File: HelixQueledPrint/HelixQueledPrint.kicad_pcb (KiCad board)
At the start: 4 copper layers, 120 parts, among them J1 USB_C_Receptacle_USB2.0_16P, J101 Conn_Coaxial, J601 Screw_Terminal_01x02, SW1 SW_SPST, SW2 SW_SPST, U101 ESP32-C6FHx, U102 BGS12WN6E6327, U202 TPS92201, U302 TPS92201, U402 TPS92201, U502 TPS92201, U601 MB34F, U602 SY8366H, U603 XBL1117, Y1 40MHz

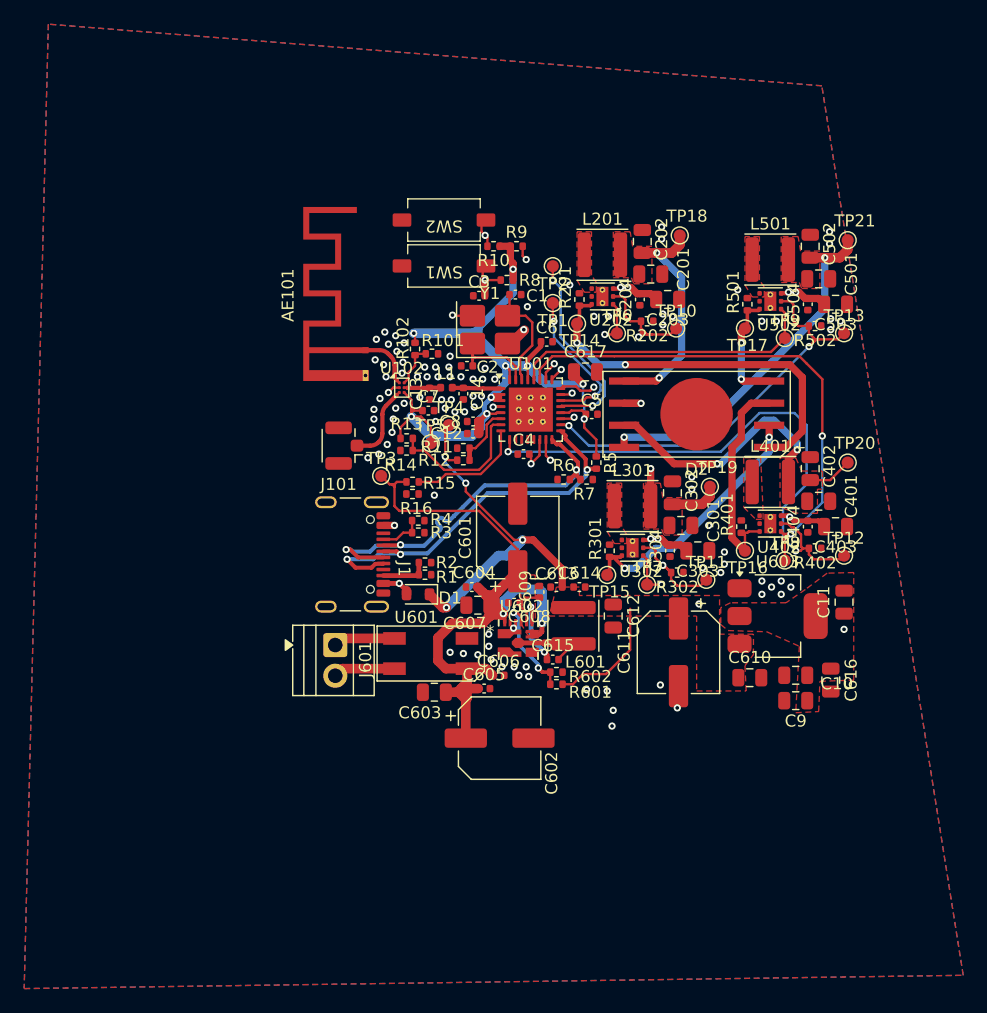
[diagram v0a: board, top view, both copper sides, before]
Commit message: Alles afgerond, geen drc errors meer
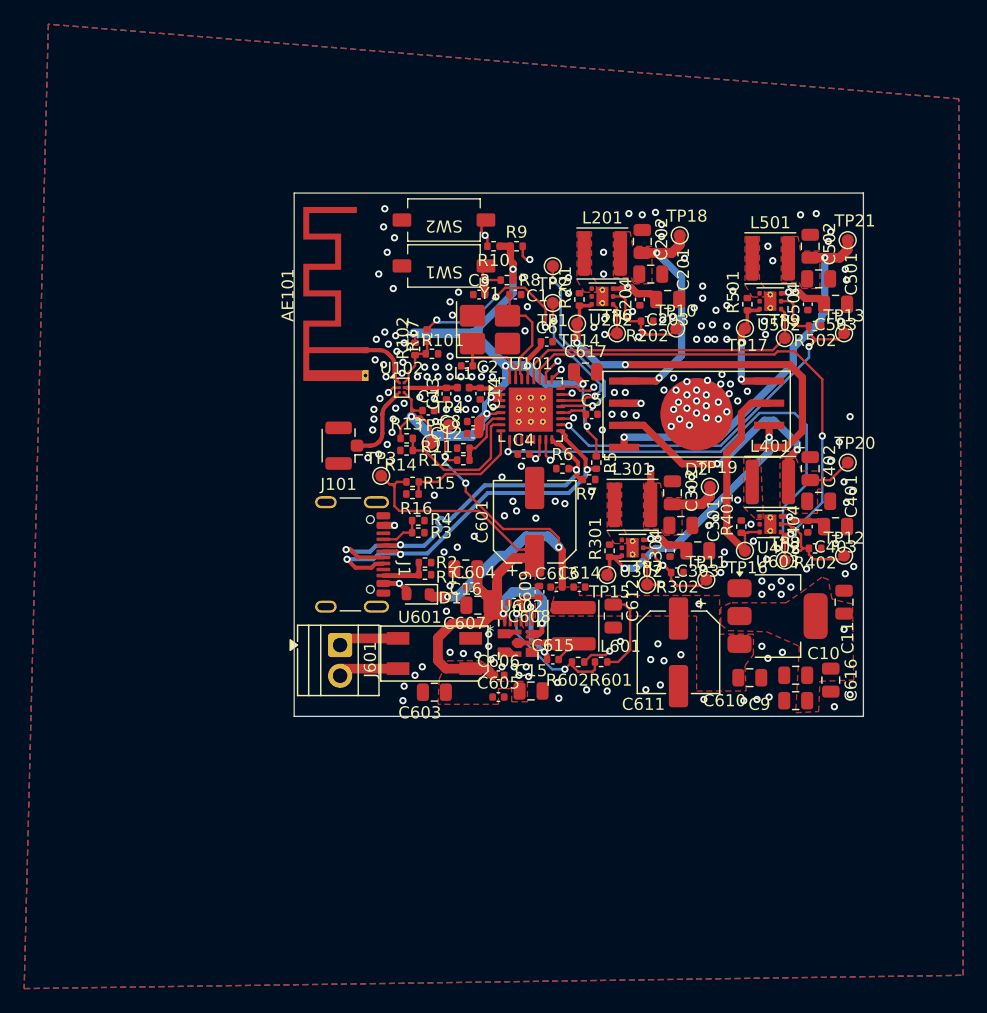
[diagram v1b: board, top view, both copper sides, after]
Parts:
- removed C602: 68uF 25V, Capacitor_SMD:CP_Elec_6.3x5.4
- added C15: 10uF 25V, Capacitor_SMD:C_0805_2012Metric, F.Cu at (124.7, 79.7)
- added C16: 10uF 25V, Capacitor_SMD:C_0805_2012Metric, F.Cu at (119.3, 69.6)
- added R17: 0R, Resistor_SMD:R_0402_1005Metric, F.Cu at (116.1, 50.3)
- moved R601 4.13 mm to (130.5, 77.3)
- moved R602 1.99 mm to (128.6, 77.3)
- moved C601 1.91 mm to (125.0, 65.7)
- moved C13 1.40 mm to (117.7, 55.1)
- moved C14 1.40 mm to (120.5, 55.1)
- moved L1 1.40 mm to (119.1, 54.6)
- moved C605 1.37 mm to (122.0, 80.2)
- moved R6 0.91 mm to (127.3, 61.3)
- moved J601 0.40 mm to (108.9, 75.9)
- moved U601 0.30 mm to (116.7, 76.6)
- moved R7 0.20 mm to (129.5, 62.2)
- moved L201 0.11 mm to (130.6, 43.5)
- moved L301 0.10 mm to (133.1, 64.3)
- moved C3 0.10 mm to (120.4, 46.9)
- moved L501 0.10 mm to (144.5, 43.9)
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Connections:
- U101 pad 19: unconnected-(U101-GPIO15-Pad19) -> /GPIO15
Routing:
- net /GPIO15: track 0.00 -> 23.8 mm, vias 0 -> 4
- net /PSU/VinDC: track 63.1 -> 57.6 mm
- net GND: track 8.16 -> 5.27 mm, vias 82 -> 208
- net Net-(U602-FB): track 8.85 -> 11.7 mm
- net /PWMG: track 27.5 -> 29.8 mm
- net /GPIO8: track 26.8 -> 24.7 mm
- net Net-(U101-ANT): track 4.03 -> 2.55 mm
- net Net-(U102-RFIN): track 3.06 -> 4.43 mm
- net +5V: track 116.3 -> 117.6 mm, vias 12 -> 11
- net unconnected-(U101-GPIO15-Pad19): track 1.16 -> 0.00 mm, vias 1 -> 0
- net /LedDriverWhite/LED+: track 30.3 -> 31.4 mm
- net /ADC1_CH2: track 9.67 -> 10.7 mm
- net Net-(U102-CTRL): track 3.60 -> 4.49 mm
- net +3V3: track 111.8 -> 112.4 mm
- net /ENW: track 34.2 -> 34.8 mm
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- added copper zone on F.Cu, net /PSU/VinDC
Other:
- board outline added: 47.1 x 43.3 mm
